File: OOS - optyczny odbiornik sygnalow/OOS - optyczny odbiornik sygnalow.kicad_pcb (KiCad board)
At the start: 2 copper layers, 72 x 78.6 mm, 126 parts, among them J1 Conn_01x02_Pin, J4 Conn_01x02_Socket, J5 Conn_Coaxial, J6 USB_C_Receptacle, Q1 SI2301CDS-T1-GE3, Q2 AOSS32334C, Q3 AOSS32334C, U1 OPA300AIDBVR, U2 OPA300AIDBVR, U3 AP3015KTR-G1, U4 MCP73831T-2ATI/OT, U5 AP9101CAK6-ANTRG1, U6 AP2126K-ADJTRG1

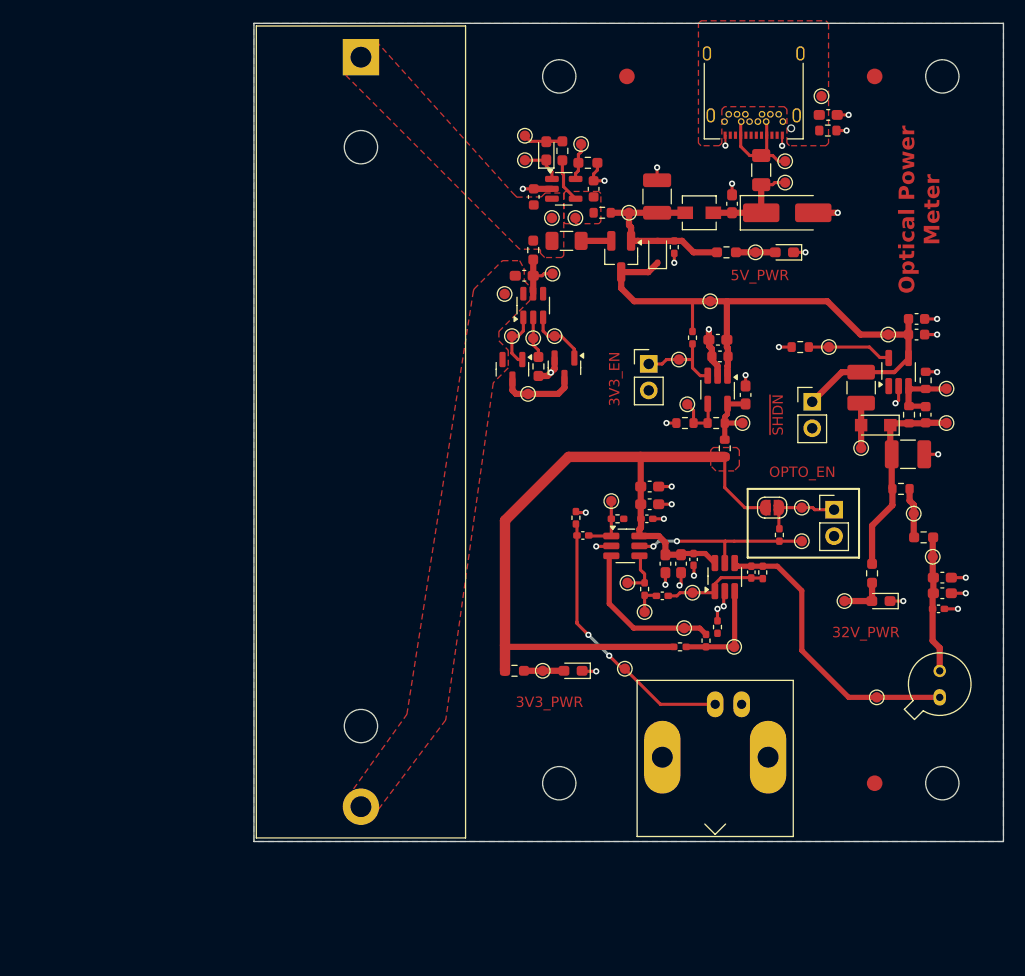
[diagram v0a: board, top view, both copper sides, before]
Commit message: Zrobiony nieco lepszy layout
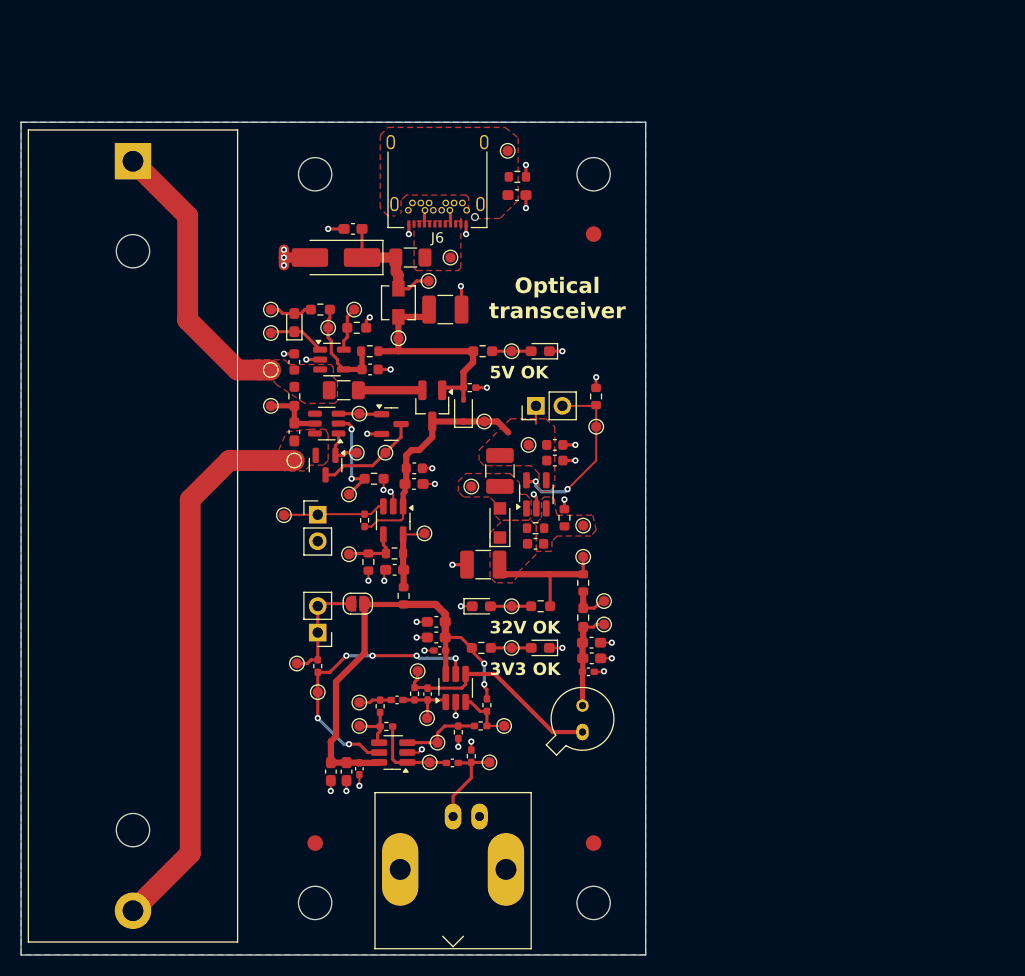
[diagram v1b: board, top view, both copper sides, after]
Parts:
- moved H2 79.5 mm to (227.9, 114.4), turned to 0 degrees
- moved FID3 78.4 mm to (227.9, 108.6), turned to 0 degrees
- moved H3 63.0 mm to (201.2, 44.4)
- moved H4 61.3 mm to (201.2, 114.4)
- moved FID1 54.1 mm to (201.2, 108.6)
- moved J4 51.0 mm to (201.4, 88.4), turned to 180 degrees
- moved TP34 50.8 mm to (199.4, 91.4)
- moved TP5 48.7 mm to (201.4, 94.1)
- moved R4 46.1 mm to (201.4, 91.6)
- moved TP6 44.2 mm to (211.0, 92.1), turned to 0 degrees
- moved D7 43.6 mm to (203.2, 52.4), turned to 180 degrees
- moved C16 42.2 mm to (217.3, 81.9), turned to 180 degrees
- moved C2 41.1 mm to (202.7, 101.8), turned to -90 degrees
- moved JP1 40.9 mm to (205.3, 85.6), turned to 0 degrees
- moved TP30 40.8 mm to (198.2, 77.1), turned to 0 degrees
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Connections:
- net Net-(D4-K) renamed /Sekcja_DCDC_Boost/D4_kathode
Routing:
- net -BAT: track 0.00 -> 53.3 mm
- net +V_DCDC_BOOST: track 59.5 -> 24.4 mm
- net +3V3: track 78.8 -> 44.2 mm, vias 0 -> 2
- net +BAT: track 0.00 -> 27.4 mm
- net /Sekcja_Analogowa/U2_x10_Out_AC: track 26.1 -> 8.95 mm, vias 2 -> 0
- net /Sekcja_Analogowa/U1/U2_En: track 17.9 -> 27.2 mm, vias 2 -> 6
- net /Sekcja_DCDC_Boost/U3_~{SHDN}: track 8.11 -> 17.2 mm, vias 0 -> 2
- net /Sekcja_USB/J6_Vbus: track 10.8 -> 2.66 mm
- net /Sekcja_DCDC_Boost/D4_kathode: track 19.8 -> 12.3 mm
- net /Sekcja_Analogowa/U2_x10_+: track 15.0 -> 7.64 mm
- net /Sekcja_DCDC_Boost/U3_FB: track 7.14 -> 0.00 mm
- net /Sekcja_Analogowa/U1_TIA_-: track 28.4 -> 21.3 mm
- net /Sekcja_Li-ion_Ladowanie/U5_VM: track 4.01 -> 10.1 mm, vias 0 -> 2
- net /Sekcja_Li-ion_Ladowanie/U3_V_{DD}: track 4.02 -> 9.97 mm
- net /Sekcja_Analogowa/U1_TIA_+: track 9.97 -> 5.47 mm
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- added copper zone on F.Cu, net +V_DCDC_BOOST
- added copper zone on F.Cu, net /Sekcja_DCDC_Boost/D4_kathode
- added copper zone on F.Cu, net /Sekcja_DCDC_Boost/U3_FB
- added copper zone on F.Cu, net /Sekcja_DCDC_Boost/U3_SW
- added copper zone on F.Cu, net /Sekcja_USB/J6_Vbus
- removed copper zone on F.Cu, net +3V3
- removed copper zone on F.Cu, net /Sekcja_Li-ion_Ladowanie/U3_V_{DD}
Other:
- board size 72 x 78.6 mm -> 60 x 80 mm
- board text added: "32V OK"
- board text added: "3V3 OK"
- board text added: "5V OK"
- board text added: "Optical transceiver"
- board text removed: "32V_PWR"
- board text removed: "3V3_EN"
- board text removed: "3V3_PWR"
- board text removed: "5V_PWR"
- board text removed: "OPTO_EN"
- board text removed: "Optical Power Meter"
- board text removed: "~{SHDN}"
